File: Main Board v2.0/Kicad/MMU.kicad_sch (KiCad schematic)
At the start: 10 parts, among them U1 GLT725608, U2 GLT725608, U3 74HC245, U4 74HC245

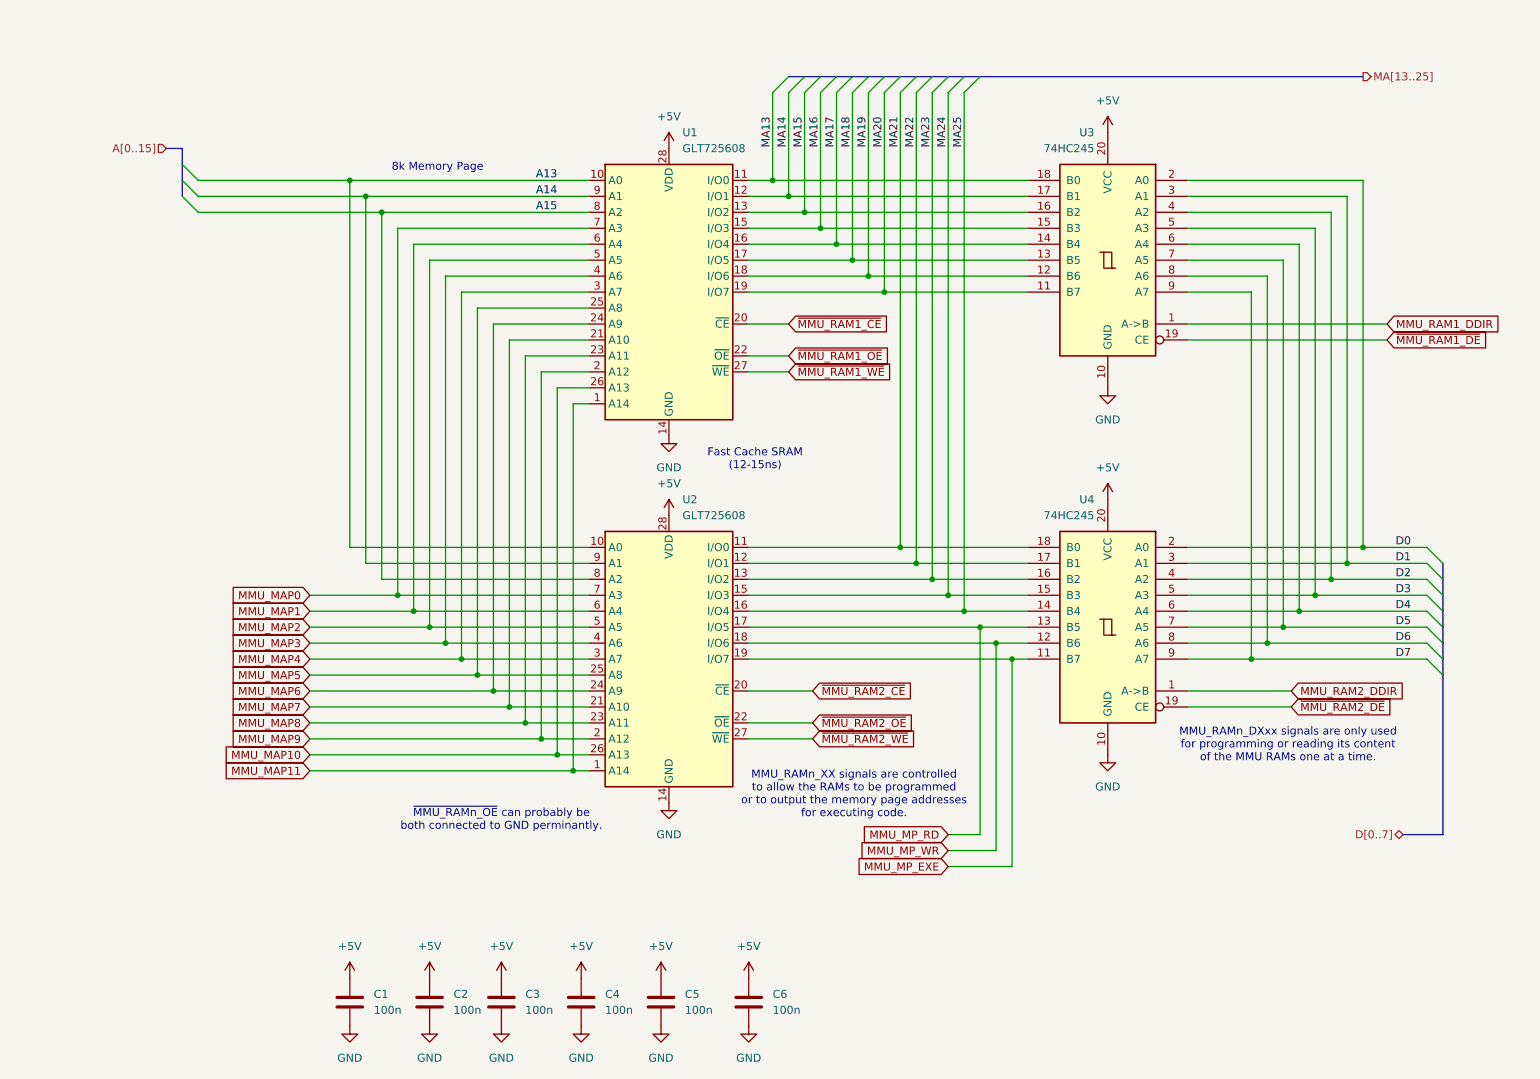
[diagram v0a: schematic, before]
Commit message: board update
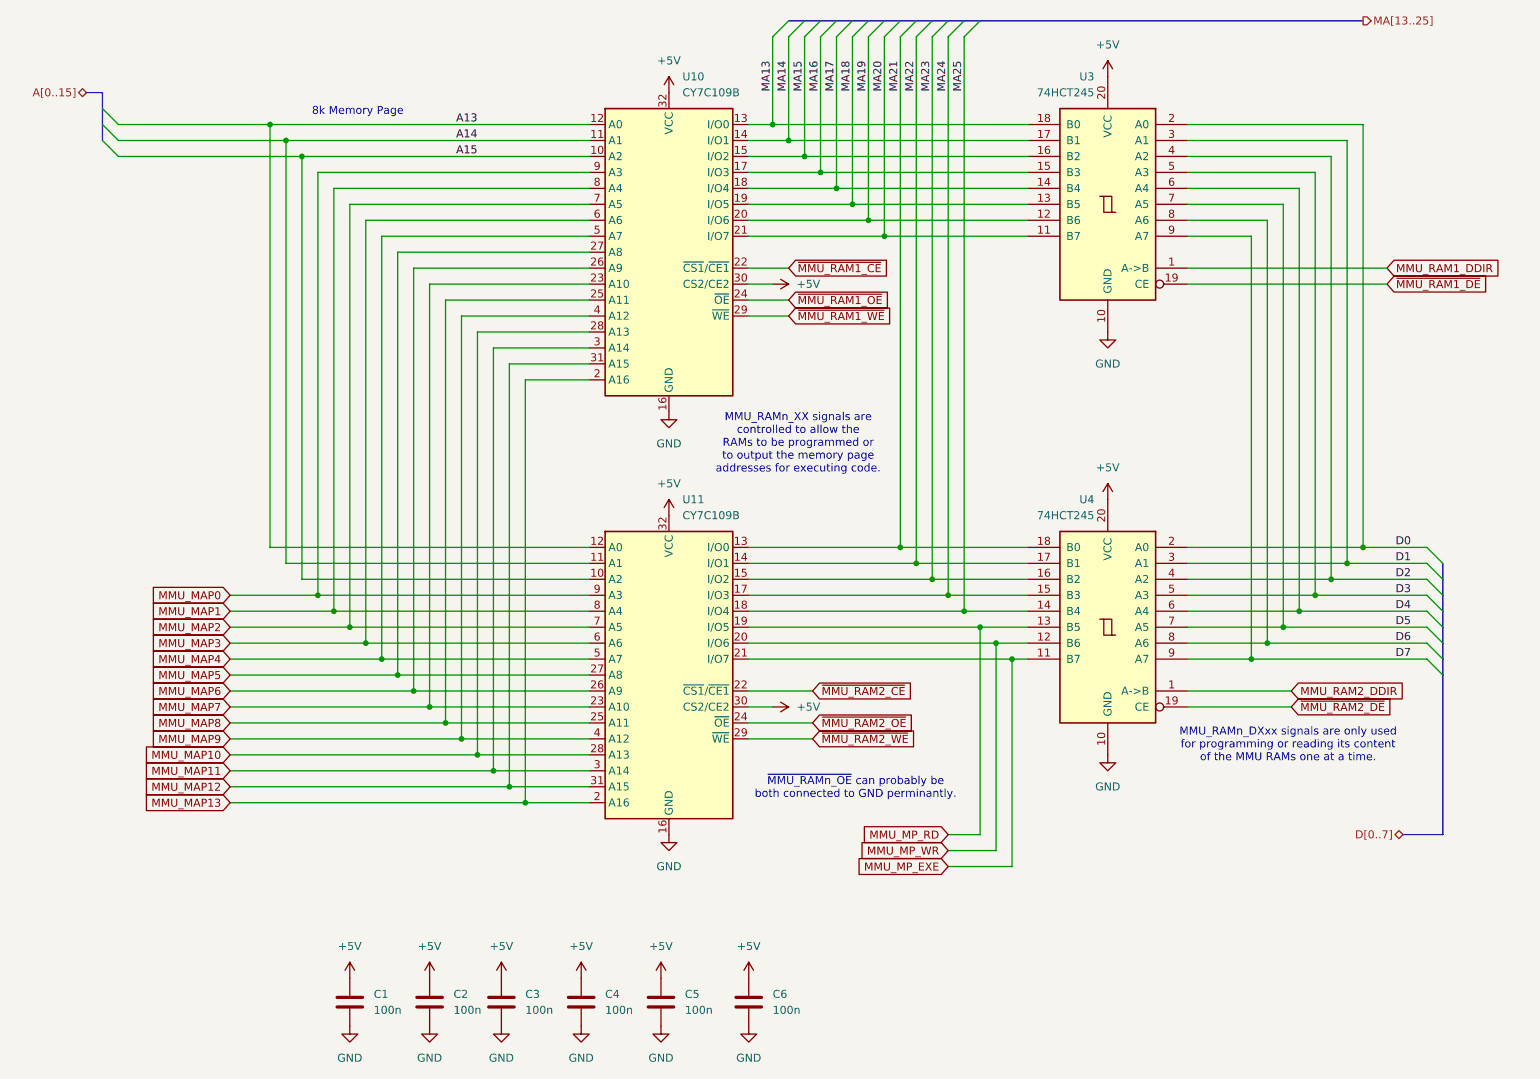
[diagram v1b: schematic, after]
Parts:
- removed U1, U2: GLT725608, Package_SO:SOJ-28_7.62x18.415mm_P1.27mm, symbol Memory_RAM:IS62C256AL
- added U10, U11: CY7C109B, Package_SO:SOJ-32_10.16x20.955mm_P1.27mm, symbol Memory_RAM:IS6xC1024AL-xxK
- U3, U4: value 74HC245 -> 74HCT245; footprint Package_SO:TSSOP-20-1EP_4.4x6.5mm_P0.65mm_EP2.15x3.35mm -> Package_DIP:CERDIP-20_W7.62mm_SideBrazed_LongPads_Socket
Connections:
- net +5V: now also U10.30 (CS2/CE2), U10.32 (VCC), U11.30 (CS2/CE2), U11.32 (VCC)
- net A13: now also U10.12 (A0), U11.12 (A0)
- net A14: now also U10.11 (A1), U11.11 (A1)
- net A15: now also U10.10 (A2), U11.10 (A2)
- net GND: now also U10.16 (GND), U11.16 (GND)
- net MA13: now also U10.13 (I/O0)
- net MA14: now also U10.14 (I/O1)
- net MA15: now also U10.15 (I/O2)
- net MA16: now also U10.17 (I/O3)
- net MA17: now also U10.18 (I/O4)
- net MA18: now also U10.19 (I/O5)
- net MA19: now also U10.20 (I/O6)
- net MA20: now also U10.21 (I/O7)
- net MA21: now also U11.13 (I/O0)
- net MA22: now also U11.14 (I/O1)
- net MA23: now also U11.15 (I/O2)
- net MA24: now also U11.17 (I/O3)
- net MA25: now also U11.18 (I/O4)
- net MMU_MAP0: now also U10.9 (A3), U11.9 (A3)
- net MMU_MAP1: now also U10.8 (A4), U11.8 (A4)
- net MMU_MAP10: now also U10.28 (A13), U11.28 (A13)
- net MMU_MAP11: now also U10.3 (A14), U11.3 (A14)
- net MMU_MAP2: now also U10.7 (A5), U11.7 (A5)
- net MMU_MAP3: now also U10.6 (A6), U11.6 (A6)
- net MMU_MAP4: now also U10.5 (A7), U11.5 (A7)
- net MMU_MAP5: now also U10.27 (A8), U11.27 (A8)
- net MMU_MAP6: now also U10.26 (A9), U11.26 (A9)
- net MMU_MAP7: now also U10.23 (A10), U11.23 (A10)
- net MMU_MAP8: now also U10.25 (A11), U11.25 (A11)
- net MMU_MAP9: now also U10.4 (A12), U11.4 (A12)
- net MMU_MP_EXE: now also U11.21 (I/O7)
- net MMU_MP_RD: now also U11.19 (I/O5)
- net MMU_MP_WR: now also U11.20 (I/O6)
- net ~{MMU_RAM1_CE}: now also U10.22 (~{CS1}/~{CE1})
- net ~{MMU_RAM1_OE}: now also U10.24 (~{OE})
- net ~{MMU_RAM1_WE}: now also U10.29 (~{WE})
- net ~{MMU_RAM2_CE}: now also U11.22 (~{CS1}/~{CE1})
- net ~{MMU_RAM2_OE}: now also U11.24 (~{OE})
- net ~{MMU_RAM2_WE}: now also U11.29 (~{WE})
- new net MMU_MAP12: U10.31 (A15), U11.31 (A15)
- new net MMU_MAP13: U10.2 (A16), U11.2 (A16)
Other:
- note removed: "Fast Cache SRAM (12-15ns)"
- moved on the sheet: U3
